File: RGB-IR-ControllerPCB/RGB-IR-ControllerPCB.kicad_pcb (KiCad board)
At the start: 2 copper layers, 63 x 63 mm, 13 parts, among them J1 Screw_Terminal_01x02, J2 Screw_Terminal_01x04, Q1 IRF540N, Q2 IRF540N, Q3 IRF540N, U1 TSOP17xx

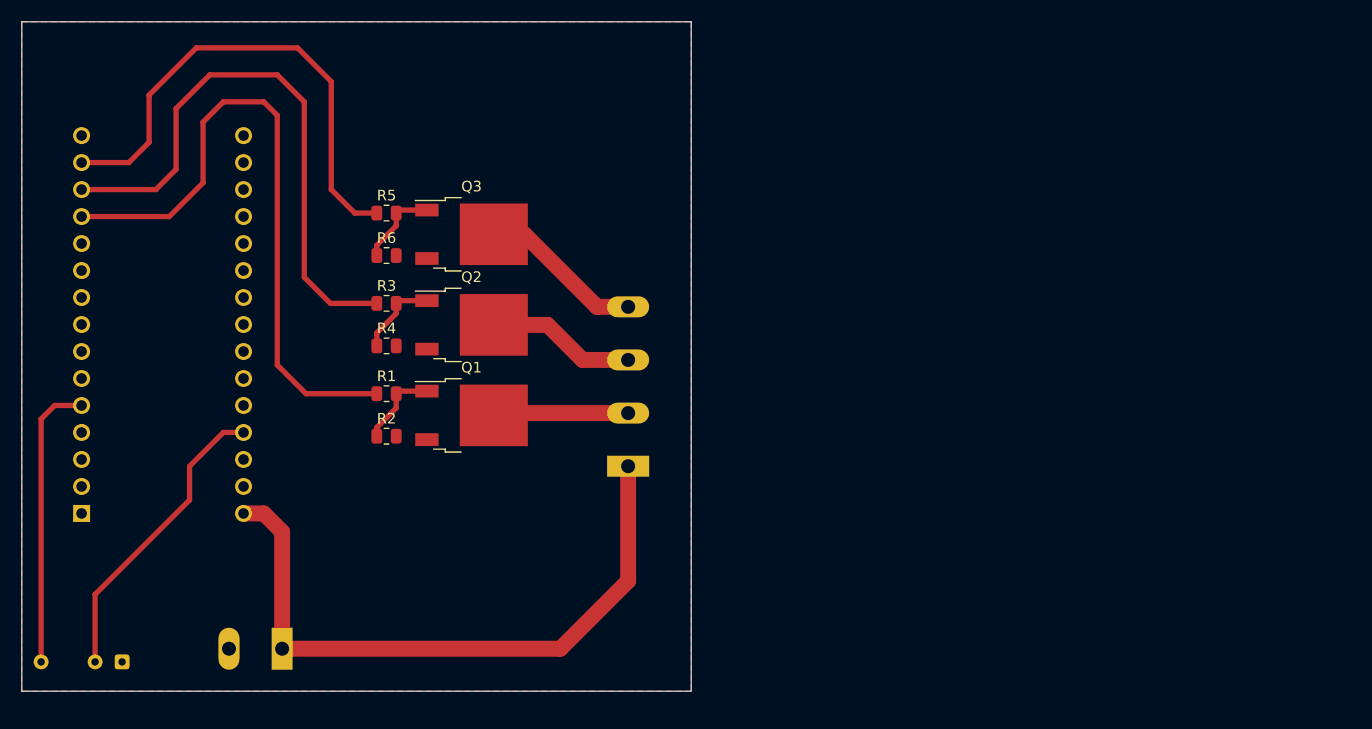
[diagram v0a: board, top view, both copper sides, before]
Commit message: Refactored PCB
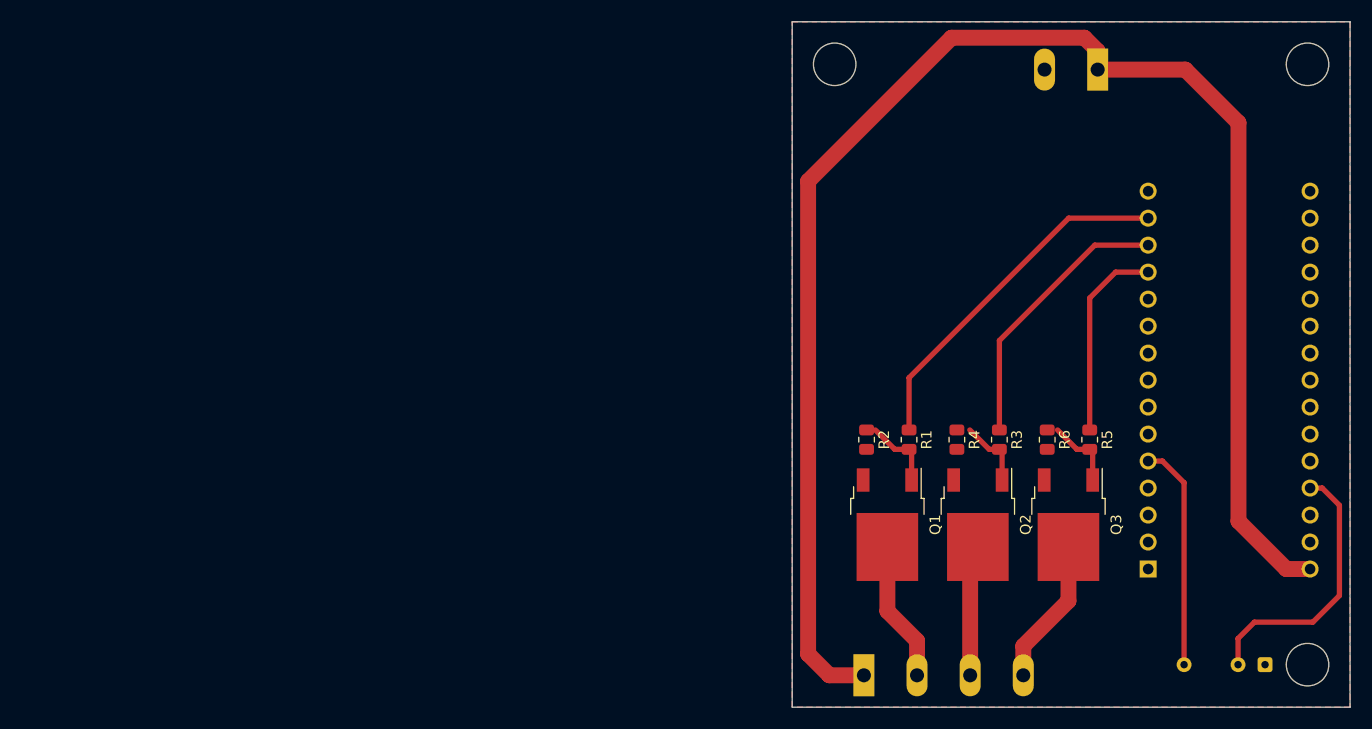
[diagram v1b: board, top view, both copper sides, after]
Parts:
- moved U1 107.6 mm to (135.5, 79.0)
- moved A1 100.5 mm to (124.5, 70.0)
- moved J1 94.1 mm to (119.8, 23.0)
- moved R5 69.5 mm to (119.0, 57.8), turned to 270 degrees
- moved R6 64.5 mm to (115.0, 57.8), turned to 270 degrees
- moved Q3 62.5 mm to (117.0, 65.8), turned to 270 degrees
- moved R3 59.1 mm to (110.5, 57.8), turned to 270 degrees
- moved R4 54.4 mm to (106.5, 57.8), turned to 270 degrees
- moved Q2 51.2 mm to (108.5, 65.8), turned to 270 degrees
- moved R1 49.4 mm to (102.0, 57.8), turned to 270 degrees
- moved R2 45.2 mm to (98.0, 57.8), turned to 270 degrees
- moved Q1 40.5 mm to (100.0, 65.8), turned to 270 degrees
- moved J2 29.7 mm to (97.8, 80.0), turned to 0 degrees
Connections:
- A1 pad 12: GREEN_PIN -> BLUE_PIN
- A1 pad 14: BLUE_PIN -> GREEN_PIN
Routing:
- net +12V: track 61.4 -> 147.1 mm
- net BLUE_PIN: track 47.2 -> 18.9 mm
- net RED_PIN: track 54.2 -> 26.1 mm
- net GREEN_PIN: track 60.7 -> 33.6 mm
- net IR_DATA_OUT: track 27.2 -> 21.3 mm
- net +5V: track 28.5 -> 25.6 mm
- net Net-(J2-Pad3): track 14.0 -> 12.4 mm
- net Net-(J2-Pad4): track 15.5 -> 13.8 mm
- net Net-(Q2-Pad1): track 7.75 -> 6.53 mm
- net Net-(Q3-Pad1): track 8.33 -> 7.35 mm
- net Net-(Q1-Pad1): track 7.74 -> 6.92 mm
- net Net-(J2-Pad2): track 15.6 -> 16.4 mm
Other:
- board size 63 x 63 mm -> 52.5 x 64.5 mm
